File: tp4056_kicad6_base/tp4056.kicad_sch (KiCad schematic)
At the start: 31 parts, among them J1 USB_B_Micro, J2 Conn_01x01_Female, J3 Conn_01x01_Female, J4 Conn_01x01_Female, J5 Conn_01x01_Female, J6 Conn_01x01_Female, J7 Conn_01x01_Female, J8 Conn_01x04_Male, Q1 FDN340P, Q2 FS8205A, U1 TP4056, U2 DW01, U3 LM1117-3.3, U4 LM809

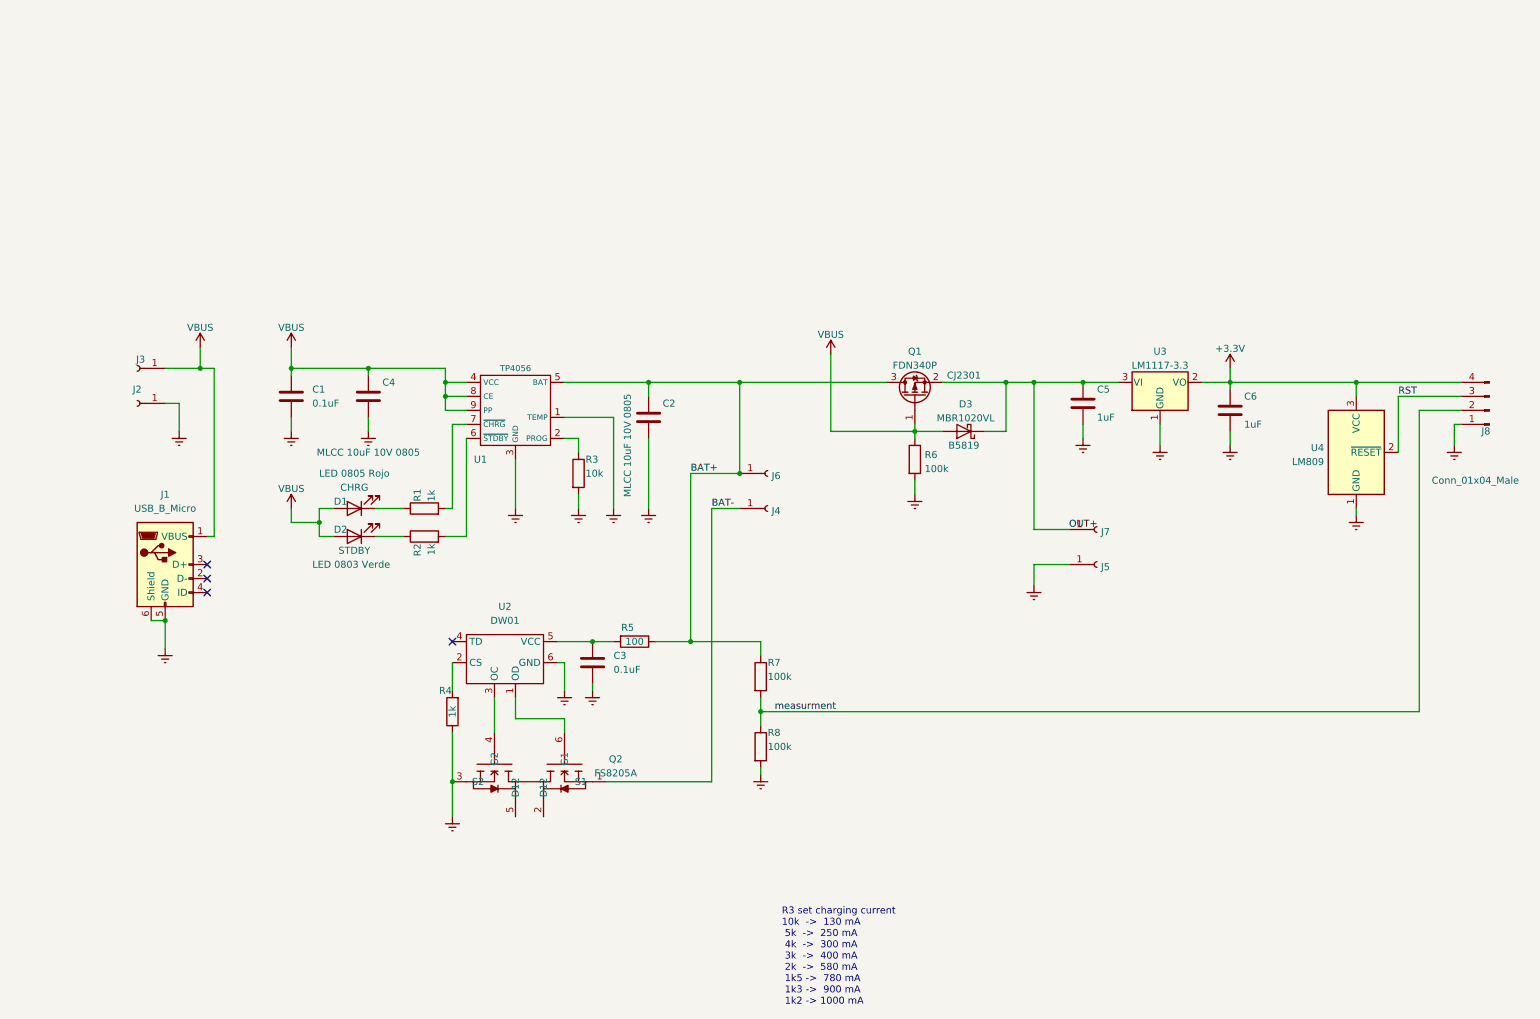
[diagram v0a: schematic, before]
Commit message: sch. redraw and organization
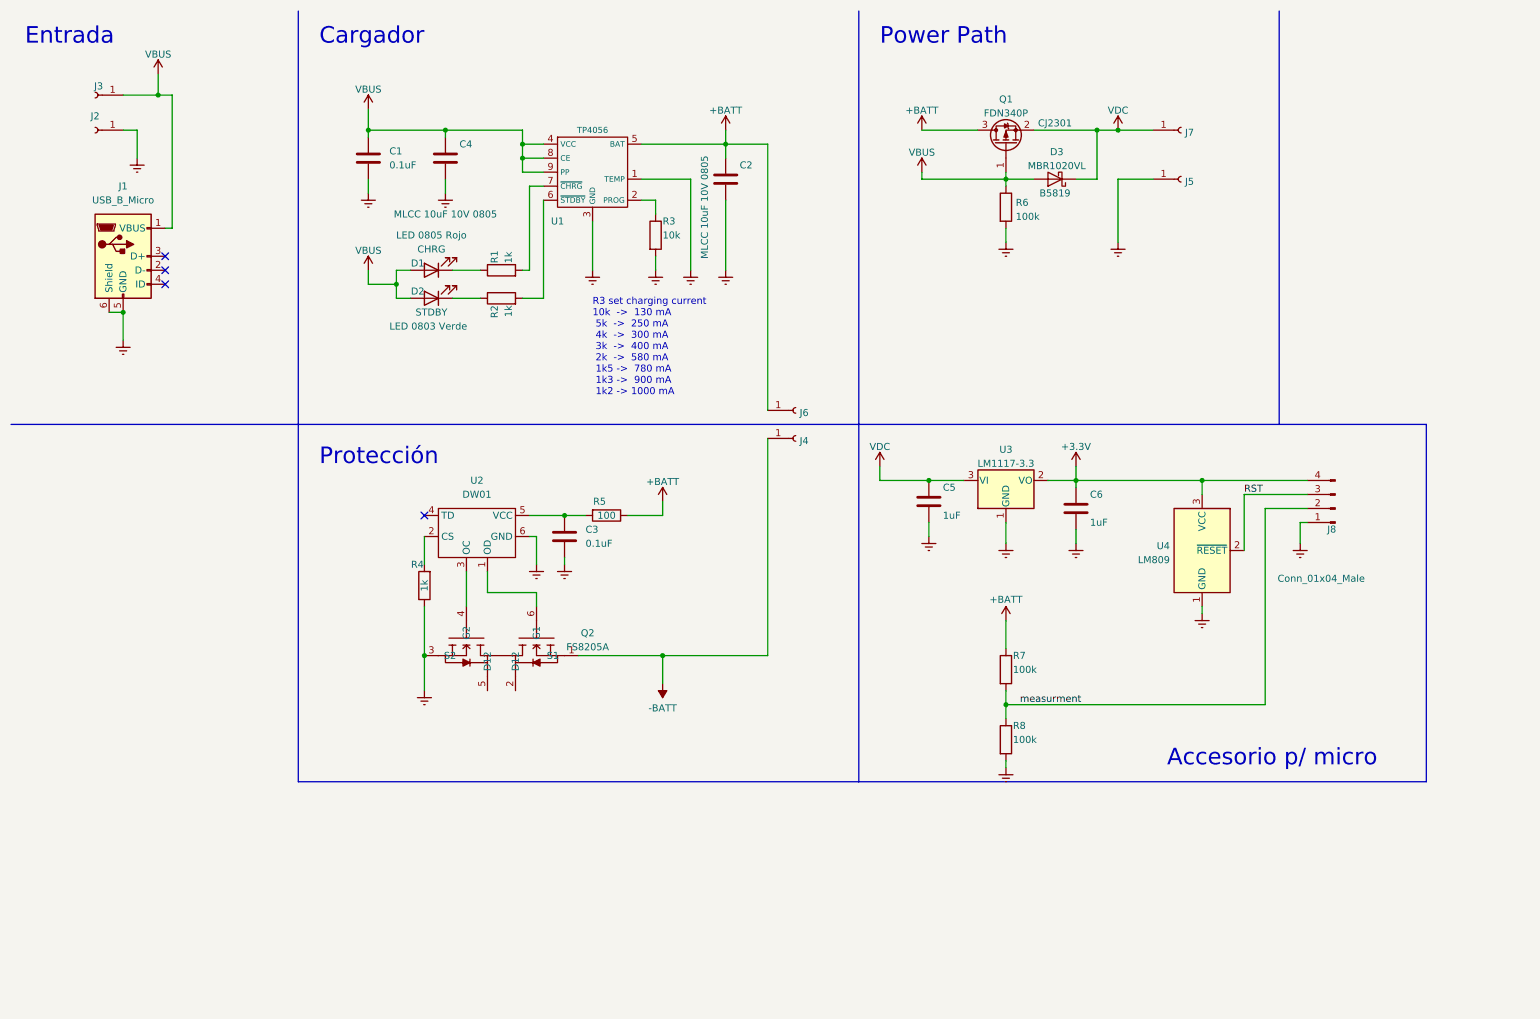
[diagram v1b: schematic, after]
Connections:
- net BAT+ renamed +BATT
- net BAT- renamed -BATT
- net OUT+ renamed VDC
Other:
- note added: "Accesorio p/ micro"
- note added: "Cargador"
- note added: "Entrada"
- note added: "Power Path"
- note added: "Protección"
- moved on the sheet: C1, C2, C3, C4, C5, C6, D1, D2, D3, J1, J2, J3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
